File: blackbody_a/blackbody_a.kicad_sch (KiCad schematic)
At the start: 27 parts, among them J1 CarPowerConnector, J2 Conn_02x04_Counter_Clockwise, SW4 SW_SPDT, SW5 SW_Push, SW6 Reset, U3 STM32L431CBTx, Y1 8M

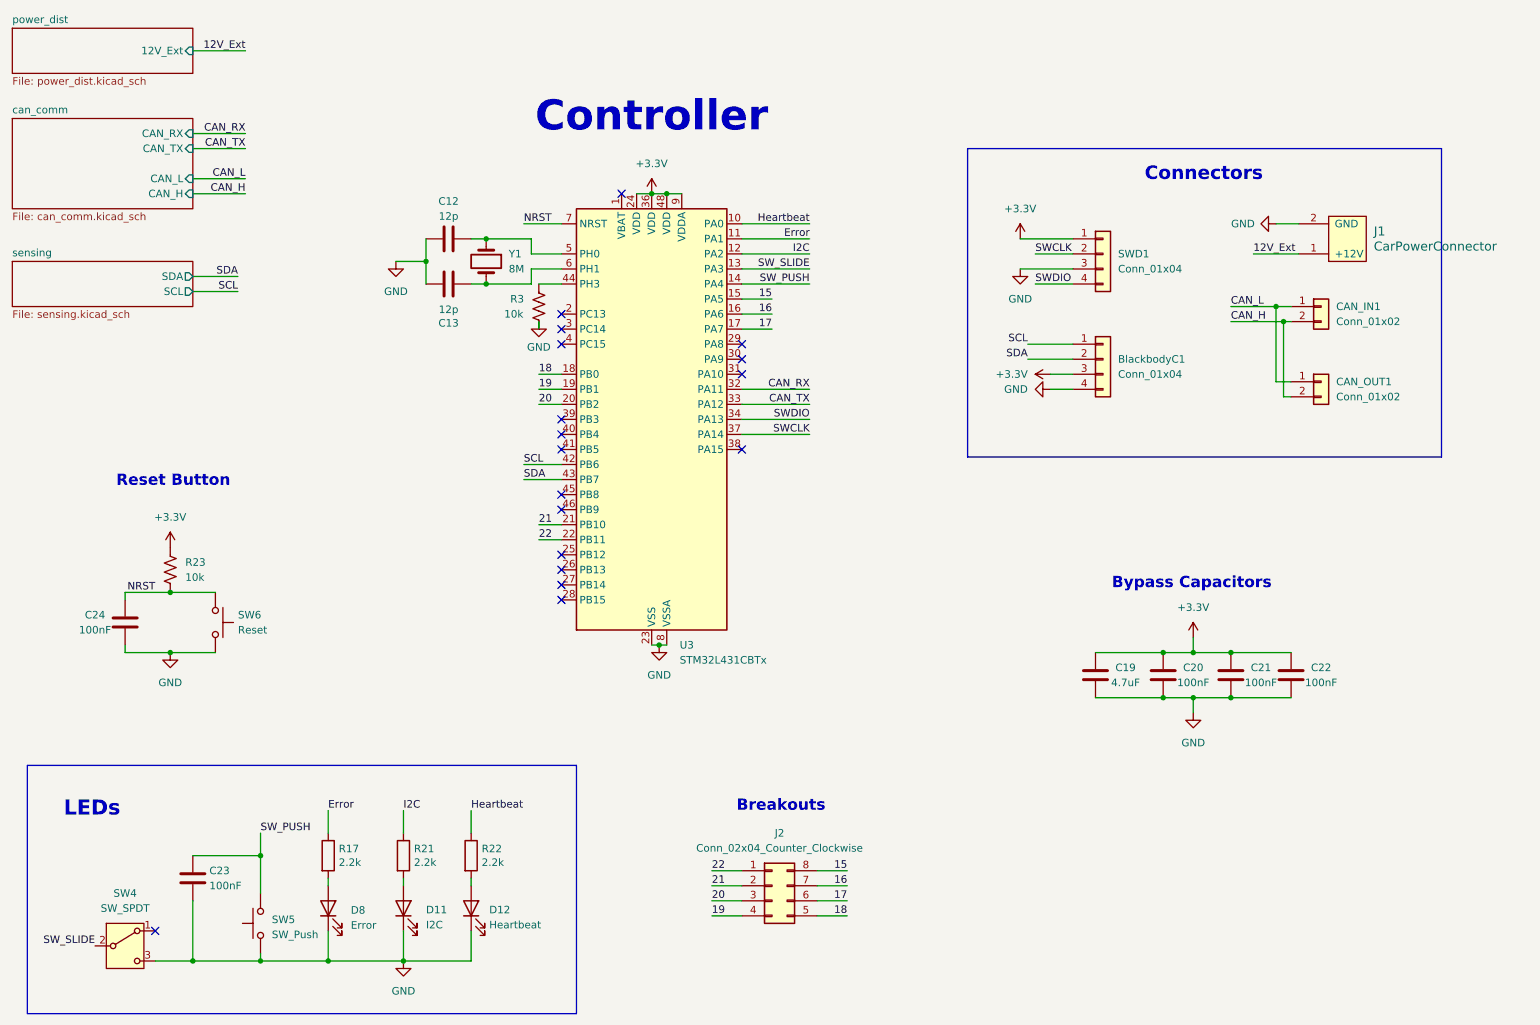
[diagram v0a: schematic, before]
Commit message: layout updates
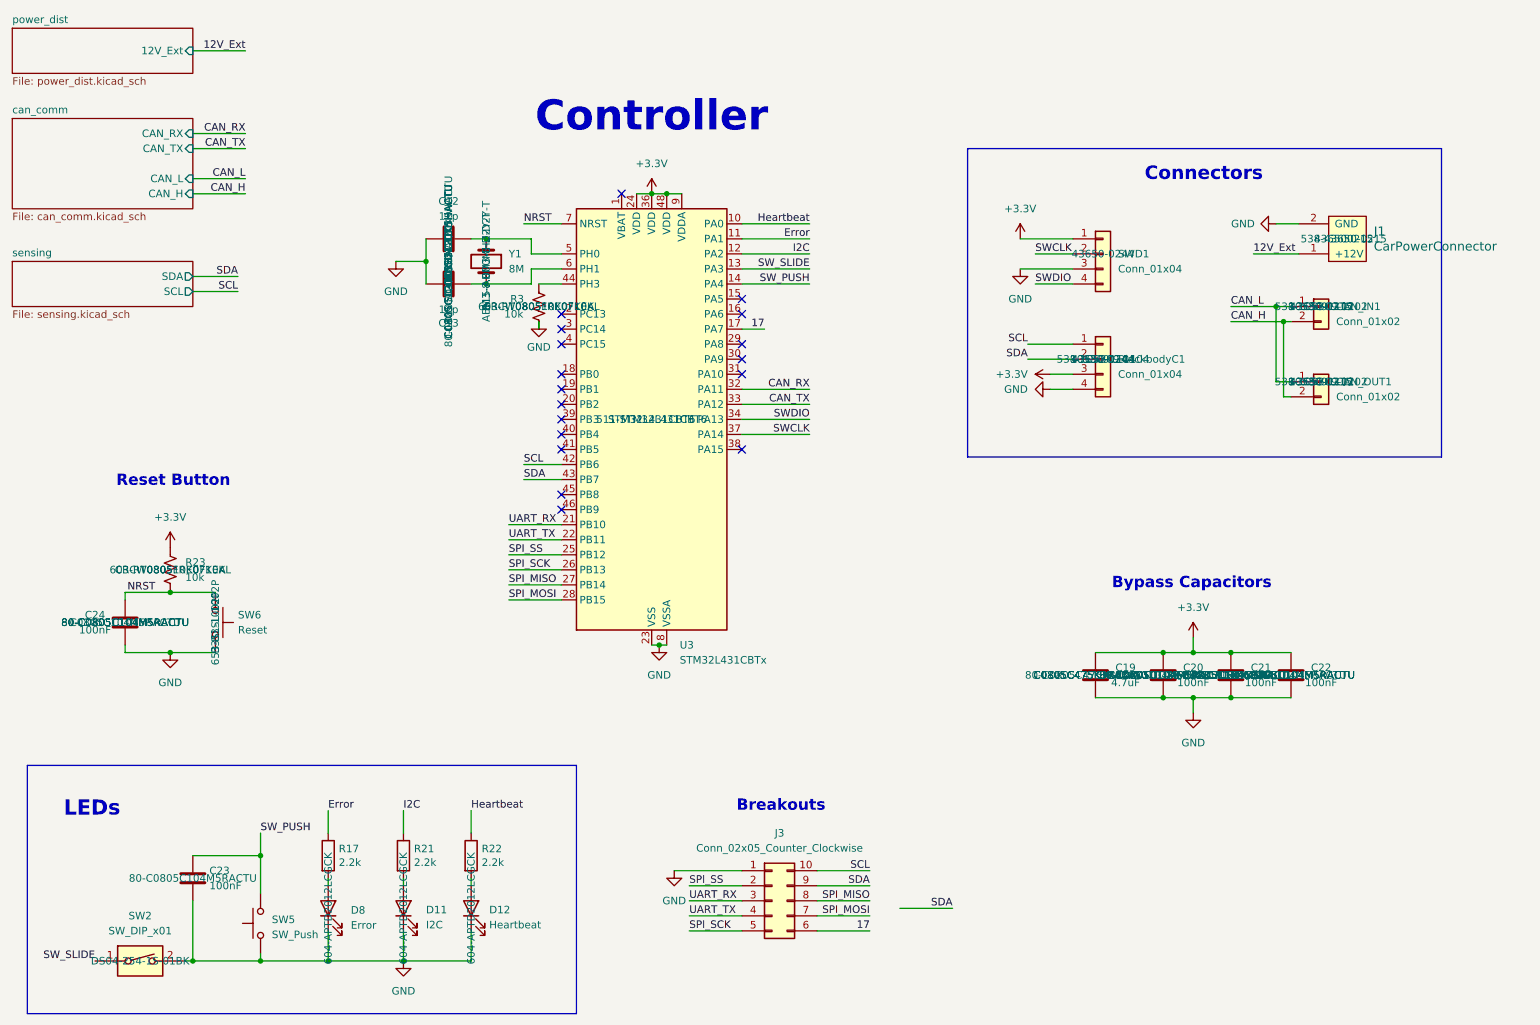
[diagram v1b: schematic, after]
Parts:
- removed J2: Conn_02x04_Counter_Clockwise, Connector_PinHeader_2.54mm:PinHeader_2x04_P2.54mm_Vertical, symbol Connector_Generic:Conn_02x04_Counter_Clockwise
- removed SW4: SW_SPDT, Button_Switch_SMD:SW_DIP_SPSTx01_Slide_6.7x4.1mm_W6.73mm_P2.54mm_LowProfile_JPin, symbol Switch:SW_SPDT
- added J3: Conn_02x05_Counter_Clockwise, Connector_PinHeader_2.54mm:PinHeader_2x05_P2.54mm_Vertical, symbol Connector_Generic:Conn_02x05_Counter_Clockwise
- added SW2: SW_DIP_x01, blackbodies:DS04254101BKSMT, symbol Switch:SW_DIP_x01
- BlackbodyC1: Manufacturer_Part_Number (none) -> 43650-0244; Mouser Part Number (none) -> 538-105309-1104; PN (none) -> 1053091104
- C12, C13: Manufacturer_Part_Number (none) -> C0805C120K5HACTU; Mouser Part Number (none) -> 80-C0805C120K5HACTU; PN (none) -> C0805C120K5HACTU
- C19: Manufacturer_Part_Number (none) -> C0805C475K3RACAUTO; Mouser Part Number (none) -> 80-C0805C475K3RACAUTO; PN (none) -> C0805C475K3RACAUTO
- C20, C21, C22, C24: Manufacturer_Part_Number (none) -> 80-C0805C104M5RACTU; Mouser Part Number (none) -> 80-C0805C104M5RACTU; PN (none) -> C0805C104M5RACTU
- C23: Manufacturer_Part_Number (none) -> 80-C0805C104M5RACTU; Mouser Part Number 80-C0805C104M5R -> 80-C0805C104M5RACTU; PN (none) -> C0805C104M5RACTU
- CAN_IN1, CAN_OUT1: Manufacturer_Part_Number (none) -> 43650-0215; Mouser Part Number (none) -> 538-105309-1102; PN (none) -> 1053091102
- D11, D12, D8: Manufacturer_Part_Number (none) -> 604-APTD2012LCGCK; PN (none) -> APTD2012LCGCK
- J1: Mouser Part Number (none) -> 538-43650-0215; PN (none) -> 436500215
- R17, R21, R22: Mouser Part Number Inventory -> 71-CRCW0805-2.2K-E3; PN (none) -> CRCW08052K20FKEA
- R23, R3: Mouser Part Number (none) -> 603-RT0805FRE0710KL; PN (none) -> CRCW080510K0FKEA
- SW5: PN (none) -> B3SL-1002P
- SW6: Mouser Part Number (none) -> 653-B3SL-1002P; PN (none) -> B3SL-1002P
- SWD1: Manufacturer_Part_Number (none) -> 43650-0244
- U3: Mouser Part Number (none) -> 511-STM32L431CBT6; PN (none) -> STM32L431CBT6
- Y1: Mouser Part Number (none) -> 815-ABM3-8-D2Y-T; PN (none) -> ABM3-8.000MHZ-D2Y-T
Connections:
- net 17: now also J3.6 (Pin_6)
- net GND: now also J3.1 (Pin_1), SW2.2
- net SCL: now also J3.10 (Pin_10)
- net SDA: now also J3.9 (Pin_9)
- net SW_SLIDE: now also SW2.1
- net SPI_SS: now reaches U3.25 (PB12)
- net SPI_SS: now also J3.2 (Pin_2)
- net SPI_SCK: now reaches U3.26 (PB13)
- net SPI_SCK: now also J3.5 (Pin_5)
- net SPI_MISO: now reaches U3.27 (PB14)
- net SPI_MISO: now also J3.8 (Pin_8)
- net SPI_MOSI: now reaches U3.28 (PB15)
- net SPI_MOSI: now also J3.7 (Pin_7)
- net 15: no longer names the net of U3.15 (PA5)
- net 16: no longer names the net of U3.16 (PA6)
- net 18: no longer names the net of U3.18 (PB0)
- net 19: no longer names the net of U3.19 (PB1)
- net 20: no longer names the net of U3.20 (PB2)
- net 21 renamed UART_RX
- net UART_RX: now also J3.3 (Pin_3)
- net 22 renamed UART_TX
- net UART_TX: now also J3.4 (Pin_4)
